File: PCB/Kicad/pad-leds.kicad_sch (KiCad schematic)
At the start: 18 parts

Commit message: fixing 3dmodels
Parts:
- PADL-D1, PADL-D2, PADL-D3, PADL-D4, PADL-D5, PADL-D6, PADL-D7, PADL-D8, PADR-D1, PADR-D2, PADR-D3, PADR-D4, PADR-D5, PADR-D6, PADR-D7, PADR-D8: footprint LED_SMD:LED_WS2812B_PLCC4_5.0x5.0mm_P3.2mm -> Library:LED_WS2812B_PLCC4_5.0x5.0mm_P3.2mm
- PADL-IN-R1, PADR-IN-R1: footprint Resistor_SMD:R_1206_3216Metric_Pad1.30x1.75mm_HandSolder -> Library:R_1206_3216Metric_Pad1.30x1.75mm_HandSolder
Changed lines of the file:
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@@
     (property "Reference" "PADL-IN-R1" (id 0) (at 43.18 68.58 90))
     (property "Value" "R_Small" (id 1) (at 43.18 73.66 90))
-    (property "Footprint" "Resistor_SMD:R_1206_3216Metric_Pad1.30x1.75mm_HandSolder" (id 2) (at 43.18 71.12 0)
+    (property "Footprint" "Library:R_1206_3216Metric_Pad1.30x1.75mm_HandSolder" (id 2) (at 43.18 71.12 0)
       (effects (font (size 1.27 1.27)) hide)
     )
@@
     (property "Reference" "PADR-IN-R1" (id 0) (at 43.18 121.92 90))
     (property "Value" "R_Small" (id 1) (at 43.18 127 90))
-    (property "Footprint" "Resistor_SMD:R_1206_3216Metric_Pad1.30x1.75mm_HandSolder" (id 2) (at 43.18 124.46 0)
+    (property "Footprint" "Library:R_1206_3216Metric_Pad1.30x1.75mm_HandSolder" (id 2) (at 43.18 124.46 0)
       (effects (font (size 1.27 1.27)) hide)
     )
@@
       (effects (font (size 1.27 1.27)) (justify left))
     )
-    (property "Footprint" "LED_SMD:LED_WS2812B_PLCC4_5.0x5.0mm_P3.2mm" (id 2) (at 57.15 78.74 0)
+    (property "Footprint" "Library:LED_WS2812B_PLCC4_5.0x5.0mm_P3.2mm" (id 2) (at 57.15 78.74 0)
       (effects (font (size 1.27 1.27)) (justify left top) hide)
     )
@@
       (effects (font (size 1.27 1.27)) (justify left))
     )
-    (property "Footprint" "LED_SMD:LED_WS2812B_PLCC4_5.0x5.0mm_P3.2mm" (id 2) (at 57.15 132.08 0)
+    (property "Footprint" "Library:LED_WS2812B_PLCC4_5.0x5.0mm_P3.2mm" (id 2) (at 57.15 132.08 0)
       (effects (font (size 1.27 1.27)) (justify left top) hide)
     )
@@
       (effects (font (size 1.27 1.27)) (justify left))
     )
-    (property "Footprint" "LED_SMD:LED_WS2812B_PLCC4_5.0x5.0mm_P3.2mm" (id 2) (at 82.55 132.08 0)
+    (property "Footprint" "Library:LED_WS2812B_PLCC4_5.0x5.0mm_P3.2mm" (id 2) (at 82.55 132.08 0)
       (effects (font (size 1.27 1.27)) (justify left top) hide)
     )
@@
       (effects (font (size 1.27 1.27)) (justify left))
     )
-    (property "Footprint" "LED_SMD:LED_WS2812B_PLCC4_5.0x5.0mm_P3.2mm" (id 2) (at 83.82 78.74 0)
+    (property "Footprint" "Library:LED_WS2812B_PLCC4_5.0x5.0mm_P3.2mm" (id 2) (at 83.82 78.74 0)
       (effects (font (size 1.27 1.27)) (justify left top) hide)
     )
@@
       (effects (font (size 1.27 1.27)) (justify left))
     )
-    (property "Footprint" "LED_SMD:LED_WS2812B_PLCC4_5.0x5.0mm_P3.2mm" (id 2) (at 108.585 132.08 0)
+    (property "Footprint" "Library:LED_WS2812B_PLCC4_5.0x5.0mm_P3.2mm" (id 2) (at 108.585 132.08 0)
       (effects (font (size 1.27 1.27)) (justify left top) hide)
     )
@@
       (effects (font (size 1.27 1.27)) (justify left))
     )
-    (property "Footprint" "LED_SMD:LED_WS2812B_PLCC4_5.0x5.0mm_P3.2mm" (id 2) (at 109.855 78.74 0)
+    (property "Footprint" "Library:LED_WS2812B_PLCC4_5.0x5.0mm_P3.2mm" (id 2) (at 109.855 78.74 0)
       (effects (font (size 1.27 1.27)) (justify left top) hide)
     )
@@
       (effects (font (size 1.27 1.27)) (justify left))
     )
-    (property "Footprint" "LED_SMD:LED_WS2812B_PLCC4_5.0x5.0mm_P3.2mm" (id 2) (at 133.985 132.08 0)
+    (property "Footprint" "Library:LED_WS2812B_PLCC4_5.0x5.0mm_P3.2mm" (id 2) (at 133.985 132.08 0)
       (effects (font (size 1.27 1.27)) (justify left top) hide)
     )
@@
       (effects (font (size 1.27 1.27)) (justify left))
     )
-    (property "Footprint" "LED_SMD:LED_WS2812B_PLCC4_5.0x5.0mm_P3.2mm" (id 2) (at 136.525 78.74 0)
+    (property "Footprint" "Library:LED_WS2812B_PLCC4_5.0x5.0mm_P3.2mm" (id 2) (at 136.525 78.74 0)
       (effects (font (size 1.27 1.27)) (justify left top) hide)
     )
@@
       (effects (font (size 1.27 1.27)) (justify left))
     )
-    (property "Footprint" "LED_SMD:LED_WS2812B_PLCC4_5.0x5.0mm_P3.2mm" (id 2) (at 158.115 132.08 0)
+    (property "Footprint" "Library:LED_WS2812B_PLCC4_5.0x5.0mm_P3.2mm" (id 2) (at 158.115 132.08 0)
       (effects (font (size 1.27 1.27)) (justify left top) hide)
     )
@@
       (effects (font (size 1.27 1.27)) (justify left))
     )
-    (property "Footprint" "LED_SMD:LED_WS2812B_PLCC4_5.0x5.0mm_P3.2mm" (id 2) (at 162.56 78.74 0)
+    (property "Footprint" "Library:LED_WS2812B_PLCC4_5.0x5.0mm_P3.2mm" (id 2) (at 162.56 78.74 0)
       (effects (font (size 1.27 1.27)) (justify left top) hide)
     )
@@
       (effects (font (size 1.27 1.27)) (justify left))
     )
-    (property "Footprint" "LED_SMD:LED_WS2812B_PLCC4_5.0x5.0mm_P3.2mm" (id 2) (at 183.515 132.08 0)
+    (property "Footprint" "Library:LED_WS2812B_PLCC4_5.0x5.0mm_P3.2mm" (id 2) (at 183.515 132.08 0)
       (effects (font (size 1.27 1.27)) (justify left top) hide)
     )
@@
       (effects (font (size 1.27 1.27)) (justify left))
     )
-    (property "Footprint" "LED_SMD:LED_WS2812B_PLCC4_5.0x5.0mm_P3.2mm" (id 2) (at 189.23 78.74 0)
+    (property "Footprint" "Library:LED_WS2812B_PLCC4_5.0x5.0mm_P3.2mm" (id 2) (at 189.23 78.74 0)
       (effects (font (size 1.27 1.27)) (justify left top) hide)
     )
@@
       (effects (font (size 1.27 1.27)) (justify left))
     )
-    (property "Footprint" "LED_SMD:LED_WS2812B_PLCC4_5.0x5.0mm_P3.2mm" (id 2) (at 209.55 132.08 0)
+    (property "Footprint" "Library:LED_WS2812B_PLCC4_5.0x5.0mm_P3.2mm" (id 2) (at 209.55 132.08 0)
       (effects (font (size 1.27 1.27)) (justify left top) hide)
     )
@@
       (effects (font (size 1.27 1.27)) (justify left))
     )
-    (property "Footprint" "LED_SMD:LED_WS2812B_PLCC4_5.0x5.0mm_P3.2mm" (id 2) (at 215.265 78.74 0)
+    (property "Footprint" "Library:LED_WS2812B_PLCC4_5.0x5.0mm_P3.2mm" (id 2) (at 215.265 78.74 0)
       (effects (font (size 1.27 1.27)) (justify left top) hide)
     )
@@
       (effects (font (size 1.27 1.27)) (justify left))
     )
-    (property "Footprint" "LED_SMD:LED_WS2812B_PLCC4_5.0x5.0mm_P3.2mm" (id 2) (at 234.95 132.08 0)
+    (property "Footprint" "Library:LED_WS2812B_PLCC4_5.0x5.0mm_P3.2mm" (id 2) (at 234.95 132.08 0)
       (effects (font (size 1.27 1.27)) (justify left top) hide)
     )
@@
       (effects (font (size 1.27 1.27)) (justify left))
     )
-    (property "Footprint" "LED_SMD:LED_WS2812B_PLCC4_5.0x5.0mm_P3.2mm" (id 2) (at 241.935 78.74 0)
-      (effects (font (size 1.27 1.27)) (justify left top) hide)
-    )
+    (property "Footprint" "Library:LED_WS2812B_PLCC4_5.0x5.0mm_P3.2mm" (id 2) (at 241.935 78.74 0)
+      (effects (font (size 1.27 1.27)) (justify left top) hide)
+    )

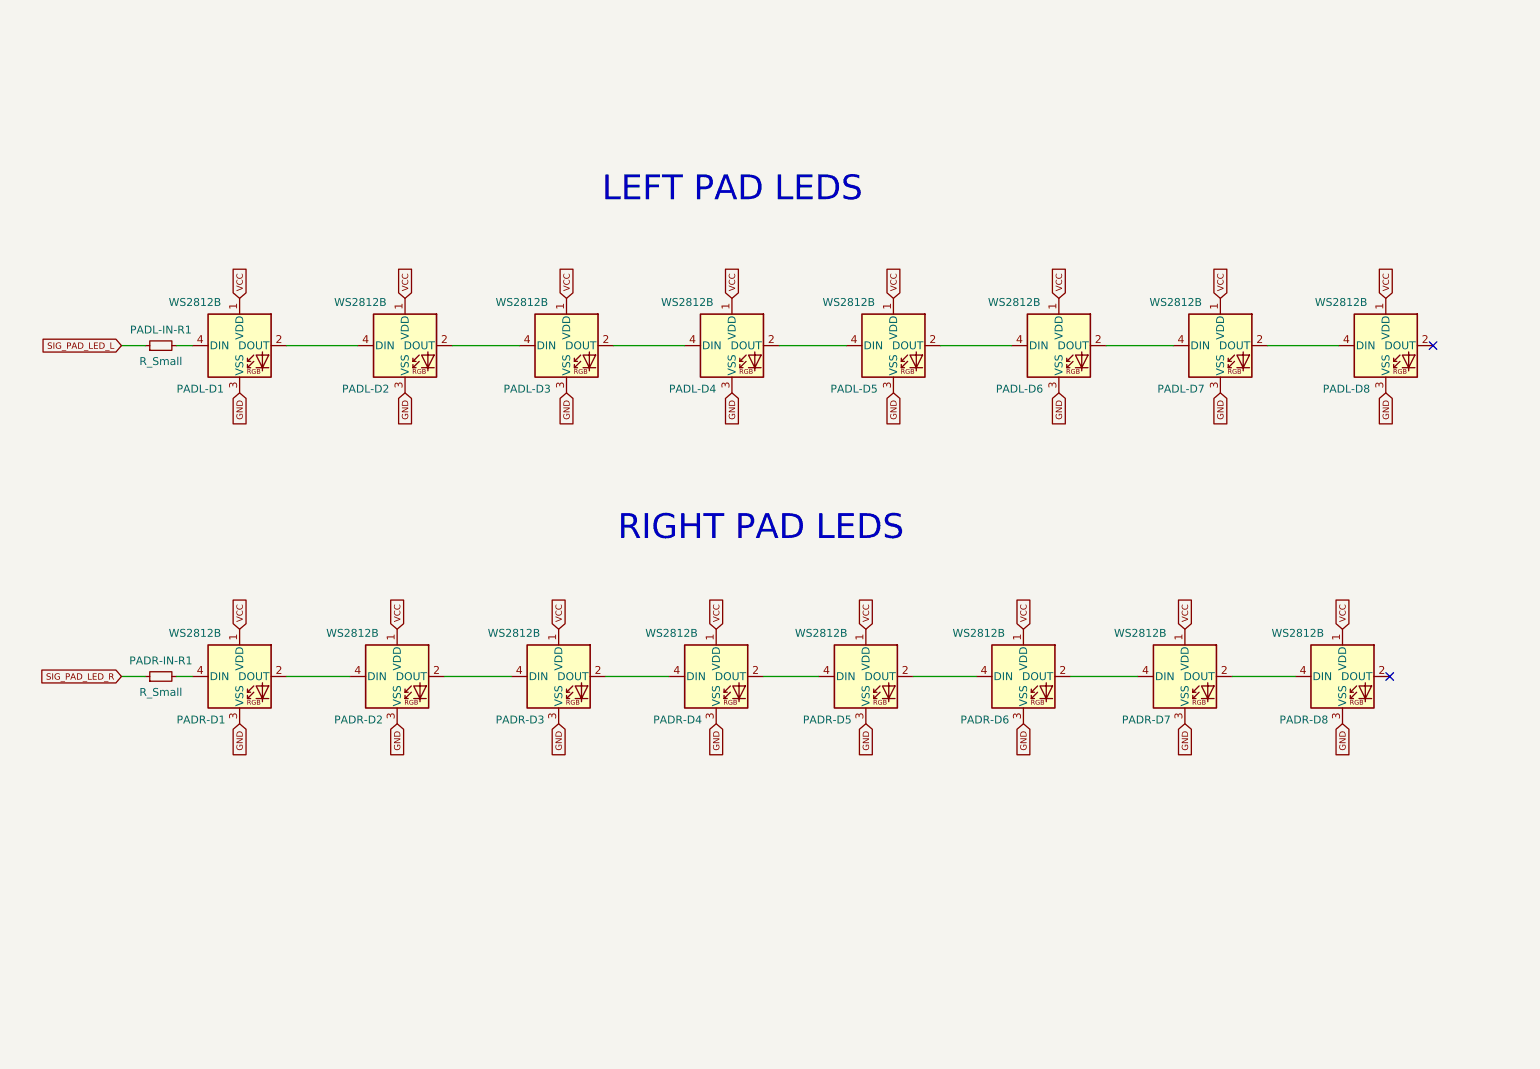
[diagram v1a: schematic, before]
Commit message: routing
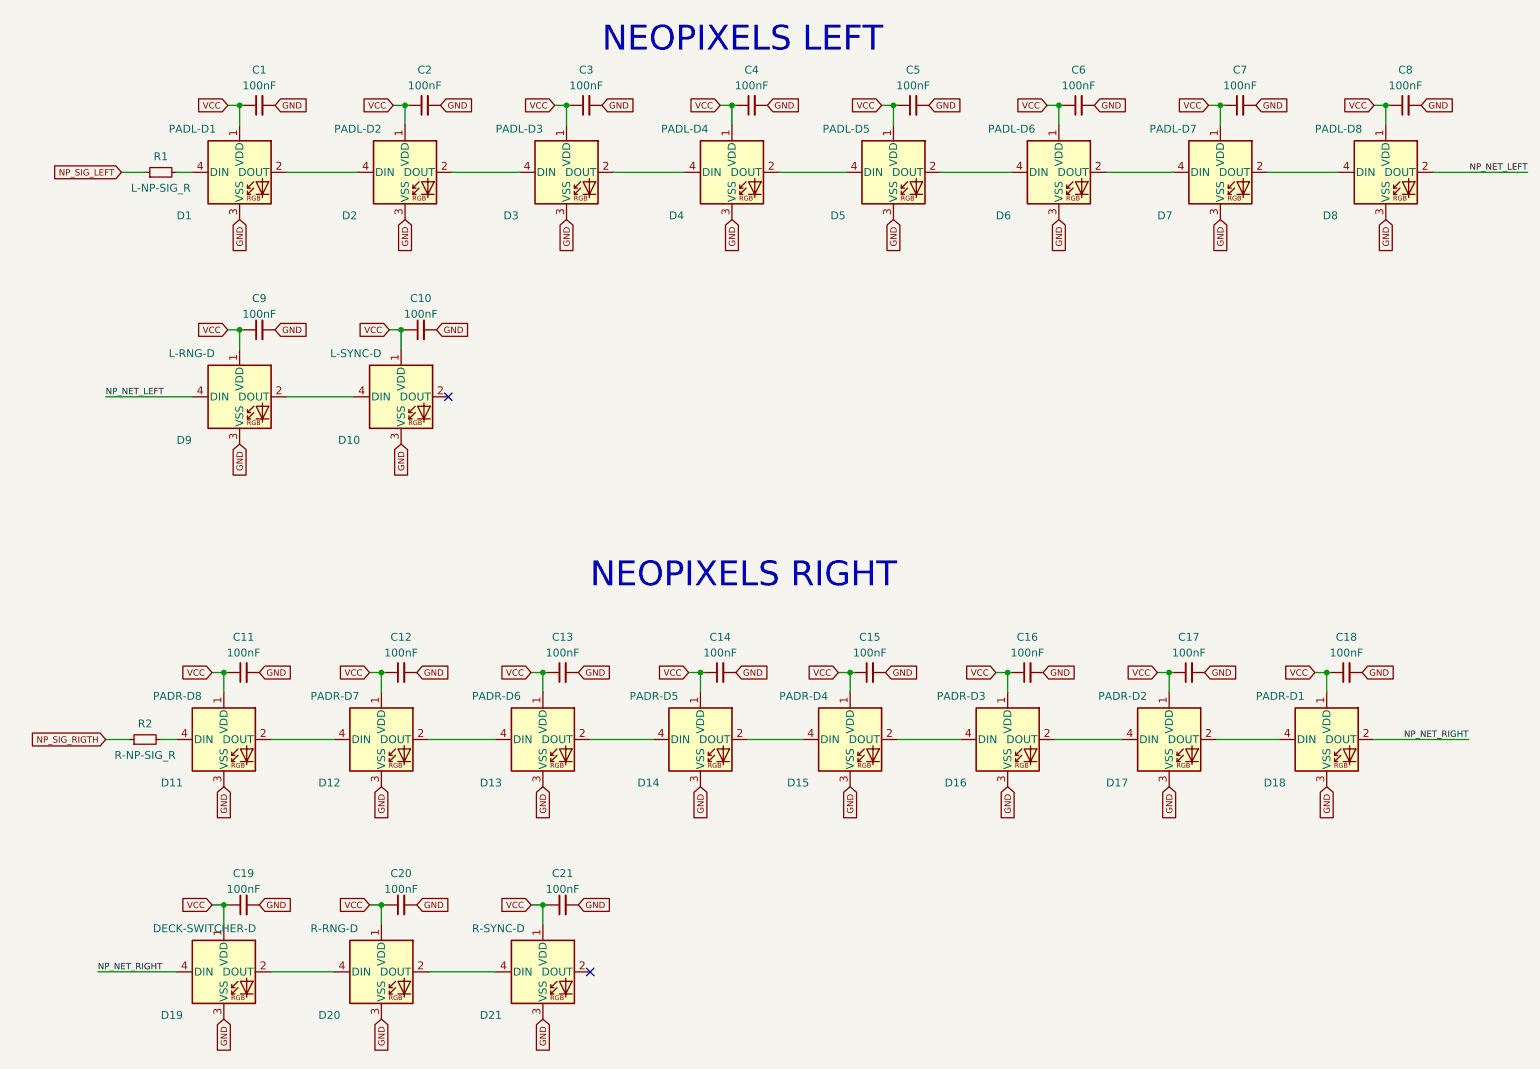
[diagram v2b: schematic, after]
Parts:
- added C1, C10, C11, C12, C13, C14, C15, C16, C17, C18, C19, C2, C20, C21, C3, C4, C5, C6, C7, C8, C9: 100nF, Capacitor_SMD:C_1206_3216Metric_Pad1.33x1.80mm_HandSolder, symbol Device:C_Small
- added D10: L-SYNC-D, LED_SMD:LED_WS2812B_PLCC4_5.0x5.0mm_P3.2mm, symbol LED:WS2812B
- added D19: DECK-SWITCHER-D, LED_SMD:LED_WS2812B_PLCC4_5.0x5.0mm_P3.2mm, symbol LED:WS2812B
- added D20: R-RNG-D, LED_SMD:LED_WS2812B_PLCC4_5.0x5.0mm_P3.2mm, symbol LED:WS2812B
- added D21: R-SYNC-D, LED_SMD:LED_WS2812B_PLCC4_5.0x5.0mm_P3.2mm, symbol LED:WS2812B
- added D9: L-RNG-D, LED_SMD:LED_WS2812B_PLCC4_5.0x5.0mm_P3.2mm, symbol LED:WS2812B
- D1: renamed from PADL-D1; value WS2812B -> PADL-D1; footprint Library:LED_WS2812B_PLCC4_5.0x5.0mm_P3.2mm -> LED_SMD:LED_WS2812B_PLCC4_5.0x5.0mm_P3.2mm
- D11: renamed from PADR-D8; value WS2812B -> PADR-D8; footprint Library:LED_WS2812B_PLCC4_5.0x5.0mm_P3.2mm -> LED_SMD:LED_WS2812B_PLCC4_5.0x5.0mm_P3.2mm
- D12: renamed from PADR-D7; value WS2812B -> PADR-D7; footprint Library:LED_WS2812B_PLCC4_5.0x5.0mm_P3.2mm -> LED_SMD:LED_WS2812B_PLCC4_5.0x5.0mm_P3.2mm
- D13: renamed from PADR-D6; value WS2812B -> PADR-D6; footprint Library:LED_WS2812B_PLCC4_5.0x5.0mm_P3.2mm -> LED_SMD:LED_WS2812B_PLCC4_5.0x5.0mm_P3.2mm
- D14: renamed from PADR-D5; value WS2812B -> PADR-D5; footprint Library:LED_WS2812B_PLCC4_5.0x5.0mm_P3.2mm -> LED_SMD:LED_WS2812B_PLCC4_5.0x5.0mm_P3.2mm
- D15: renamed from PADR-D4; value WS2812B -> PADR-D4; footprint Library:LED_WS2812B_PLCC4_5.0x5.0mm_P3.2mm -> LED_SMD:LED_WS2812B_PLCC4_5.0x5.0mm_P3.2mm
- D16: renamed from PADR-D3; value WS2812B -> PADR-D3; footprint Library:LED_WS2812B_PLCC4_5.0x5.0mm_P3.2mm -> LED_SMD:LED_WS2812B_PLCC4_5.0x5.0mm_P3.2mm
- D17: renamed from PADR-D2; value WS2812B -> PADR-D2; footprint Library:LED_WS2812B_PLCC4_5.0x5.0mm_P3.2mm -> LED_SMD:LED_WS2812B_PLCC4_5.0x5.0mm_P3.2mm
- D18: renamed from PADR-D1; value WS2812B -> PADR-D1; footprint Library:LED_WS2812B_PLCC4_5.0x5.0mm_P3.2mm -> LED_SMD:LED_WS2812B_PLCC4_5.0x5.0mm_P3.2mm
- D2: renamed from PADL-D2; value WS2812B -> PADL-D2; footprint Library:LED_WS2812B_PLCC4_5.0x5.0mm_P3.2mm -> LED_SMD:LED_WS2812B_PLCC4_5.0x5.0mm_P3.2mm
- D3: renamed from PADL-D3; value WS2812B -> PADL-D3; footprint Library:LED_WS2812B_PLCC4_5.0x5.0mm_P3.2mm -> LED_SMD:LED_WS2812B_PLCC4_5.0x5.0mm_P3.2mm
- D4: renamed from PADL-D4; value WS2812B -> PADL-D4; footprint Library:LED_WS2812B_PLCC4_5.0x5.0mm_P3.2mm -> LED_SMD:LED_WS2812B_PLCC4_5.0x5.0mm_P3.2mm
- D5: renamed from PADL-D5; value WS2812B -> PADL-D5; footprint Library:LED_WS2812B_PLCC4_5.0x5.0mm_P3.2mm -> LED_SMD:LED_WS2812B_PLCC4_5.0x5.0mm_P3.2mm
- D6: renamed from PADL-D6; value WS2812B -> PADL-D6; footprint Library:LED_WS2812B_PLCC4_5.0x5.0mm_P3.2mm -> LED_SMD:LED_WS2812B_PLCC4_5.0x5.0mm_P3.2mm
- D7: renamed from PADL-D7; value WS2812B -> PADL-D7; footprint Library:LED_WS2812B_PLCC4_5.0x5.0mm_P3.2mm -> LED_SMD:LED_WS2812B_PLCC4_5.0x5.0mm_P3.2mm
- D8: renamed from PADL-D8; value WS2812B -> PADL-D8; footprint Library:LED_WS2812B_PLCC4_5.0x5.0mm_P3.2mm -> LED_SMD:LED_WS2812B_PLCC4_5.0x5.0mm_P3.2mm
- R1: renamed from PADL-IN-R1; value R_Small -> L-NP-SIG_R
- R2: renamed from PADR-IN-R1; value R_Small -> R-NP-SIG_R
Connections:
- net GND: now also C1.2, C10.2, C11.2, C12.2, C13.2, C14.2, C15.2, C16.2, C17.2, C18.2, C19.2, C2.2, C20.2, C21.2, C3.2, C4.2, C5.2, C6.2, C7.2, C8.2, C9.2, D10.3 (VSS), D19.3 (VSS), D20.3 (VSS), D21.3 (VSS), D9.3 (VSS)
- net VCC: now also C1.1, C10.1, C11.1, C12.1, C13.1, C14.1, C15.1, C16.1, C17.1, C18.1, C19.1, C2.1, C20.1, C21.1, C3.1, C4.1, C5.1, C6.1, C7.1, C8.1, C9.1, D10.1 (VDD), D19.1 (VDD), D20.1 (VDD), D21.1 (VDD), D9.1 (VDD)
- net at D13.2 (DOUT): now also D14.4 (DIN); no longer D12.4 (DIN)
- net at D13.4 (DIN): now also D12.2 (DOUT); no longer D14.2 (DOUT)
- net at D16.2 (DOUT): now also D17.4 (DIN); no longer D15.4 (DIN)
- net at D16.4 (DIN): now also D15.2 (DOUT); no longer D17.2 (DOUT)
- net at R2.2: now also D11.4 (DIN); no longer D18.4 (DIN)
- net NP_NET_RIGHT: now reaches D18.2 (DOUT)
- net NP_NET_RIGHT: now also D19.4 (DIN); no longer D17.4 (DIN)
- net at D11.2 (DOUT): now also D12.4 (DIN)
- net NP_NET_LEFT: now reaches D8.2 (DOUT)
- net NP_NET_LEFT: now also D9.4 (DIN)
- net SIG_PAD_LED_L renamed NP_SIG_LEFT
- net SIG_PAD_LED_R renamed NP_SIG_RIGTH
- new net: D19.2 (DOUT), D20.4 (DIN)
- new net: D10.4 (DIN), D9.2 (DOUT)
- new net: D20.2 (DOUT), D21.4 (DIN)
- new net: D14.2 (DOUT), D15.4 (DIN)
- new net: D17.2 (DOUT), D18.4 (DIN)
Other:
- note added: "NEOPIXELS LEFT"
- note added: "NEOPIXELS RIGHT"
- note removed: "LEFT PAD LEDS"
- note removed: "RIGHT PAD LEDS"
- moved on the sheet: D1, D11, D12, D13, D14, D15, D16, D17, D18, D2, D3, D4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
